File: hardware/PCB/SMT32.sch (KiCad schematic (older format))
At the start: 26 parts, among them J1 473460001, SW1 B3U-1000P, SW2 B3U-1000P, U3 AZ1117CH-3.3TRG1, U4 STM32F303CCT6, Y1 8Mhz20pF

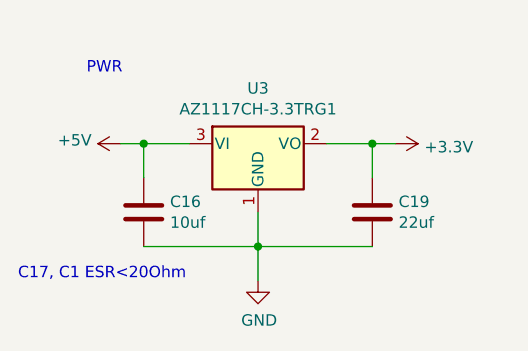
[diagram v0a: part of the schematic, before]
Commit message: attempt to remove some extra values
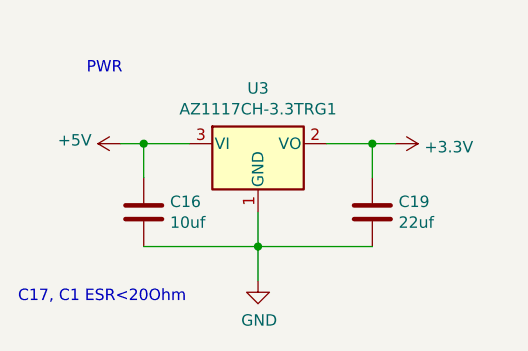
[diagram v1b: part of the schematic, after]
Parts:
- C15, C17, C18, C20, C21, C24: Footprint Capacitor_SMD:C_0402_1005Metric -> (none); Value 100nf -> (none)
- C16, C19: Footprint Capacitor_SMD:C_0402_1005Metric -> (none); Value 10uf -> (none)
- C22, C23: Footprint Capacitor_SMD:C_0402_1005Metric -> (none); Value 20pf -> (none)
- R10, R14: Footprint Resistor_SMD:R_0402_1005Metric -> (none); Value 100k -> (none)
- R11: Footprint Resistor_SMD:R_0402_1005Metric -> (none); Value 1k -> (none)
- R12, R13: Footprint Resistor_SMD:R_0402_1005Metric -> (none); Value 22 -> (none)
- R15, R16: Footprint Resistor_SMD:R_0402_1005Metric -> (none); Value 10k -> (none)
- R17, R18: Footprint Resistor_SMD:R_0402_1005Metric -> (none); Value 0 -> (none)
- R9: Footprint Resistor_SMD:R_0402_1005Metric -> (none); Value 1.5k -> (none)
- U3: Footprint Package_TO_SOT_SMD:SOT-223-3_TabPin2 -> (none); Value AS1117-3.3 -> (none)
- U4: Footprint Package_QFP:LQFP-48_7x7mm_P0.5mm -> (none); Value STM32F303CCT6 -> (none)
- Y1: Footprint Crystal:Crystal_SMD_5032-2Pin_5.0x3.2mm -> (none); P/N (none) -> X50328MSB2GI; Value X50328MSB2GI -> (none)
